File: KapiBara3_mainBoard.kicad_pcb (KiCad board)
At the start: 4 copper layers, 127.5 x 127.5 mm, 85 parts, among them J1 Conn_02x20_Top_Bottom, J2 Conn_02x20_Top_Bottom, J3 Conn_02x20_Top_Bottom, J4 Conn_02x20_Top_Bottom, J5 Conn_02x20_Top_Bottom, J6 Conn_01x02, J7 Conn_01x08, J8 Conn_01x02, J9 Conn_01x02, Q1 Q_PMOS_GDS, Q2 2N7002, Q3 Q_PMOS_GDS, U1 SL2.1A, U2 AP63300WU-7, U3 ADS1115IDGS, Y1 12Mhz

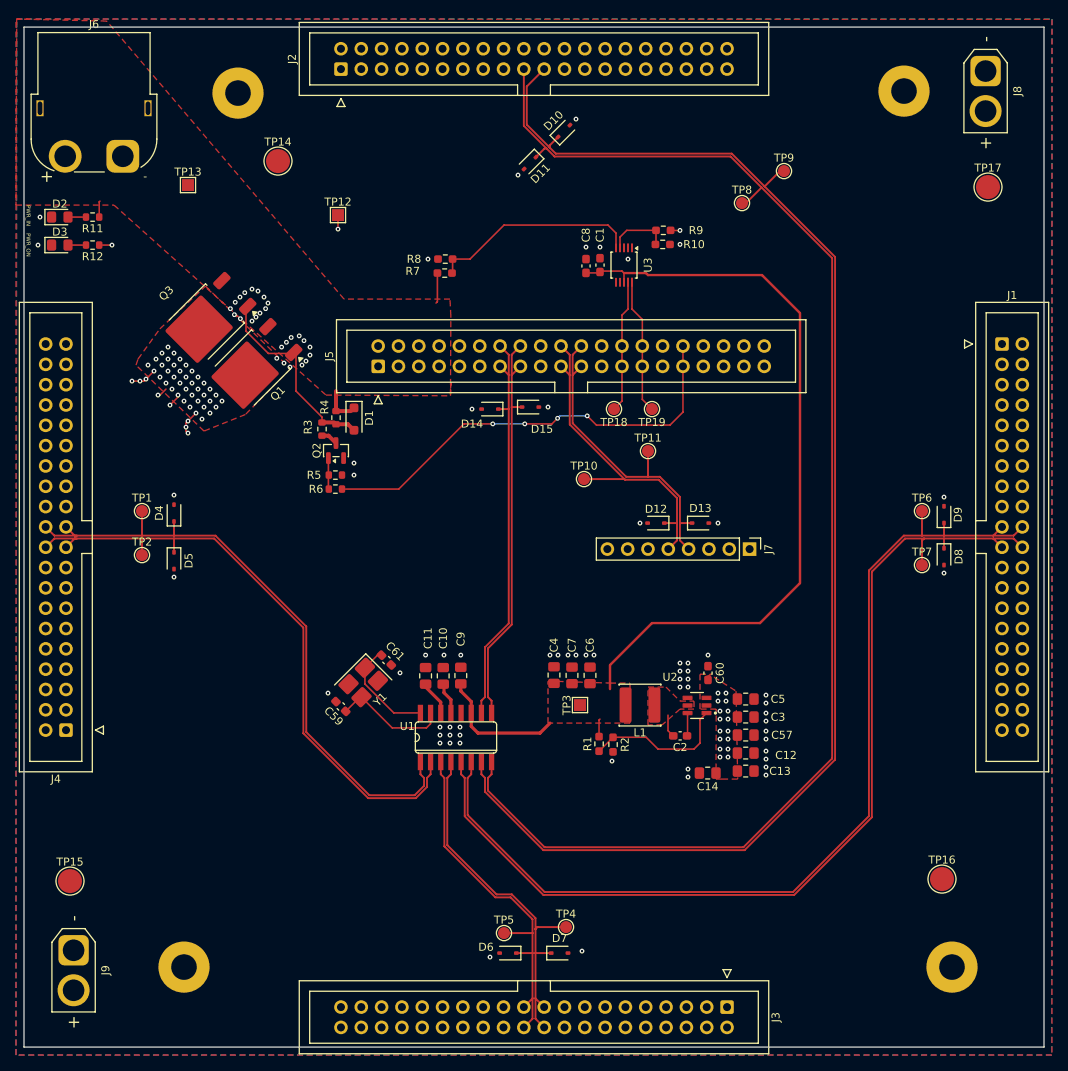
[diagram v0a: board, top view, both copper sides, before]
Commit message: I have shrinken down the board
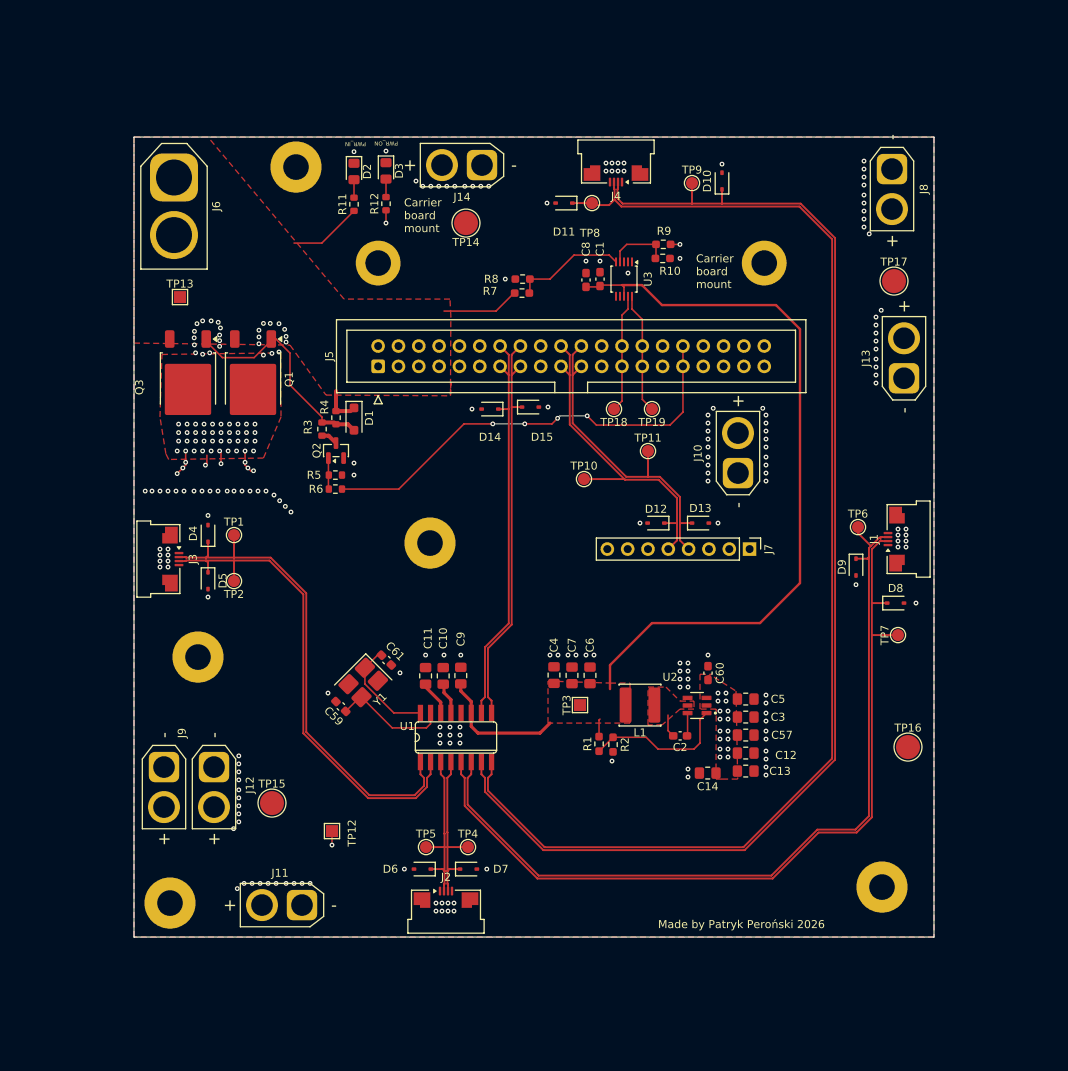
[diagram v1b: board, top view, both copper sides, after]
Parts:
- removed the REF** at (111.0, 9.00)
- added ?: , , F.Cu at (93.5, 31.0)
- added J10: Conn_01x02, Connector_AMASS:AMASS_XT30U-F_1x02_P5.0mm_Vertical, F.Cu at (90.2, 56.8)
- added J11: Conn_01x02, Connector_AMASS:AMASS_XT30U-F_1x02_P5.0mm_Vertical, F.Cu at (35.8, 110.8)
- added J12: Conn_01x02, Connector_AMASS:AMASS_XT30U-F_1x02_P5.0mm_Vertical, F.Cu at (24.8, 93.5)
- added J13: Conn_01x02, Connector_AMASS:AMASS_XT30U-F_1x02_P5.0mm_Vertical, F.Cu at (111.0, 44.9)
- added J14: Conn_01x02, Connector_AMASS:AMASS_XT30U-F_1x02_P5.0mm_Vertical, F.Cu at (58.2, 18.2)
- added REF**: MountingHole_3.2mm_M3_Pad, MountingHole:MountingHole_3.2mm_M3_Pad, F.Cu at (22.8, 79.8)
- added REF**: MountingHole_3.2mm_M3_Pad, MountingHole:MountingHole_3.2mm_M3_Pad, F.Cu at (51.8, 65.5)
- added REF**: MountingHole_3.2mm_M3_DIN965_Pad, MountingHole:MountingHole_3.2mm_M3_DIN965_Pad, F.Cu at (45.2, 30.5)
- J1, J2, J3, J4: value Conn_02x20_Top_Bottom -> Conn_01x04_MountingPin; footprint Connector_IDC:IDC-Header_2x20_P2.54mm_Vertical -> Connector_FFC-FPC:Amphenol_F32Q-1A7x1-11004_1x04-1MP_P0.5mm_Horizontal
- J6: footprint Connector_AMASS:AMASS_XT60PW-F_1x02_P7.20mm_Horizontal -> Connector_AMASS:AMASS_XT60-M_1x02_P7.20mm_Vertical
- moved J2 106.5 mm to (53.8, 111.9), turned to 0 degrees
- moved J4 99.1 mm to (75.0, 17.5)
- moved J3 90.7 mm to (17.5, 67.5)
- moved TP12 77.0 mm to (39.5, 101.5)
- moved D3 41.8 mm to (46.2, 19.0), turned to -90 degrees
- moved D2 37.2 mm to (42.2, 19.1), turned to -90 degrees
- moved R12 37.0 mm to (46.2, 23.1), turned to 90 degrees
- moved R11 32.7 mm to (42.2, 23.1), turned to 90 degrees
- moved TP15 27.1 mm to (32.0, 98.0)
- moved J1 26.9 mm to (111.9, 65.0), turned to 90 degrees
- moved J9 25.5 mm to (18.5, 93.5)
- moved TP14 24.7 mm to (56.2, 25.5), turned to 180 degrees
- moved D10 20.7 mm to (88.2, 20.2), turned to 90 degrees
- moved TP8 18.8 mm to (72.0, 23.0)
- moved TP16 17.0 mm to (111.5, 91.0)
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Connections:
- J1 pad 1: VCC -> GND
- J1 pad 2: VCC -> D3-
- J1 pad 3: VCC -> D3+
- J1 pad 4: VCC -> GND
- J2 pad 1: VCC -> GND
- J2 pad 2: VCC -> D2-
- J2 pad 3: VCC -> D2+
- J2 pad 4: VCC -> GND
- J3 pad 1: VCC -> GND
- J3 pad 2: VCC -> D1-
- J3 pad 3: VCC -> D1+
- J3 pad 4: VCC -> GND
- J4 pad 1: VCC -> GND
- J4 pad 2: VCC -> D4-
- J4 pad 3: VCC -> D4+
- J4 pad 4: VCC -> GND
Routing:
- net D2+: track 47.4 -> 20.6 mm
- net D2-: track 46.6 -> 20.5 mm
- net D4-: track 176.4 -> 156.2 mm
- net D3+: track 123.2 -> 103.6 mm
- net D3-: track 123.8 -> 104.7 mm
- net D4+: track 174.4 -> 156.2 mm
- net D1-: track 79.2 -> 61.7 mm
- net D1+: track 78.8 -> 61.5 mm
- net VDD: track 10.8 -> 23.9 mm
- net Net-(U3-AIN1): track 26.2 -> 14.1 mm
- net Net-(D1-A): track 25.0 -> 28.6 mm
- net SCL: track 17.4 -> 15.1 mm
- net SDA: track 17.1 -> 14.8 mm
- net +5V: track 113.7 -> 112.2 mm
- net GND: vias 89 -> 211
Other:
- board size 127.5 x 127.5 mm -> 100 x 100 mm
- board text added: "Carrier board mount"
- board text added: "Made by Patryk Peroński 2026"
